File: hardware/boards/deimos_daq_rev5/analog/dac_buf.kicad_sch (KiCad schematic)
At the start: 4 parts, among them IC53001 INA826AIDR

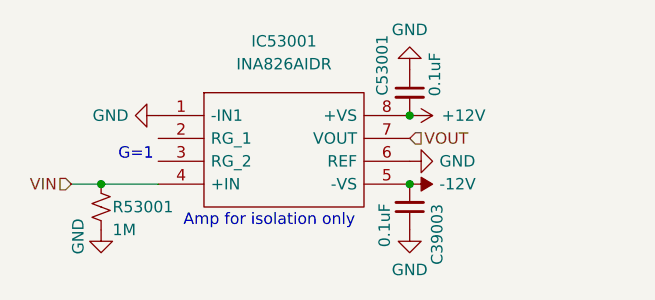
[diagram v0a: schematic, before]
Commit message: restore rev5 and make this rev rev6
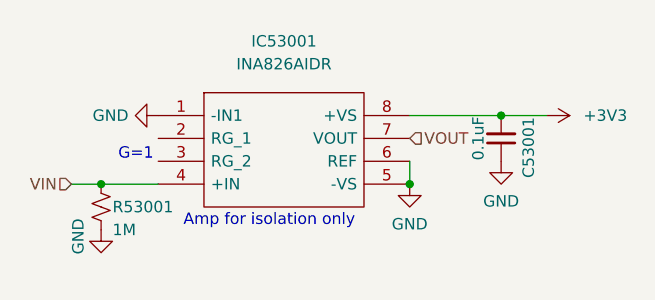
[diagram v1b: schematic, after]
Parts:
- removed C39003: 0.1uF, Capacitor_SMD:C_0402_1005Metric, symbol Device:C_Small
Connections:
- net -12V is gone; now on net GND: IC53001.5 (-VS)
- net +12V renamed +3V3
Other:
- moved on the sheet: C53001
